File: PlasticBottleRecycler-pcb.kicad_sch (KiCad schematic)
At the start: 26 parts, among them J1 SWIM, J2 LCD, J3 Screw_Terminal_01x04, J4 NTC, J5 HEATER, J6 FAN1, J7 +12V, J8 +5V, Q1 IRF3205, Q2 BC337, SW1 RESET, SW2 SW_Push, SW3 SW_Push, SW4 SW_Push, U1 STM8S005K6T6C

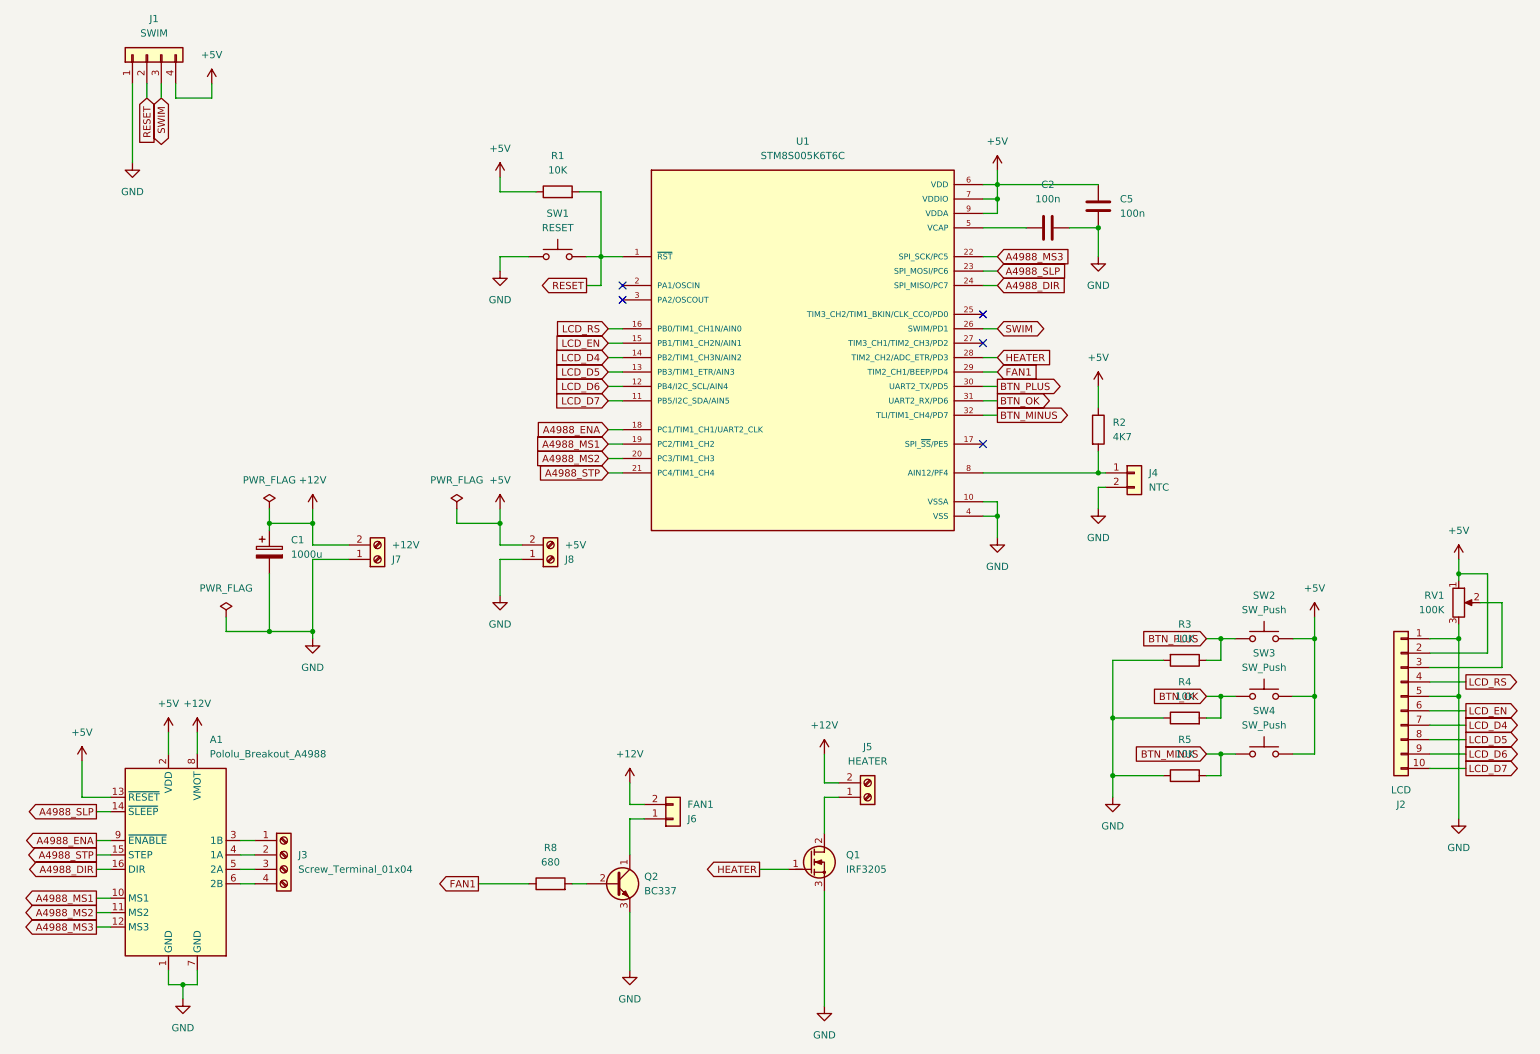
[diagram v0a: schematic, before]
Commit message: Revision 2.0
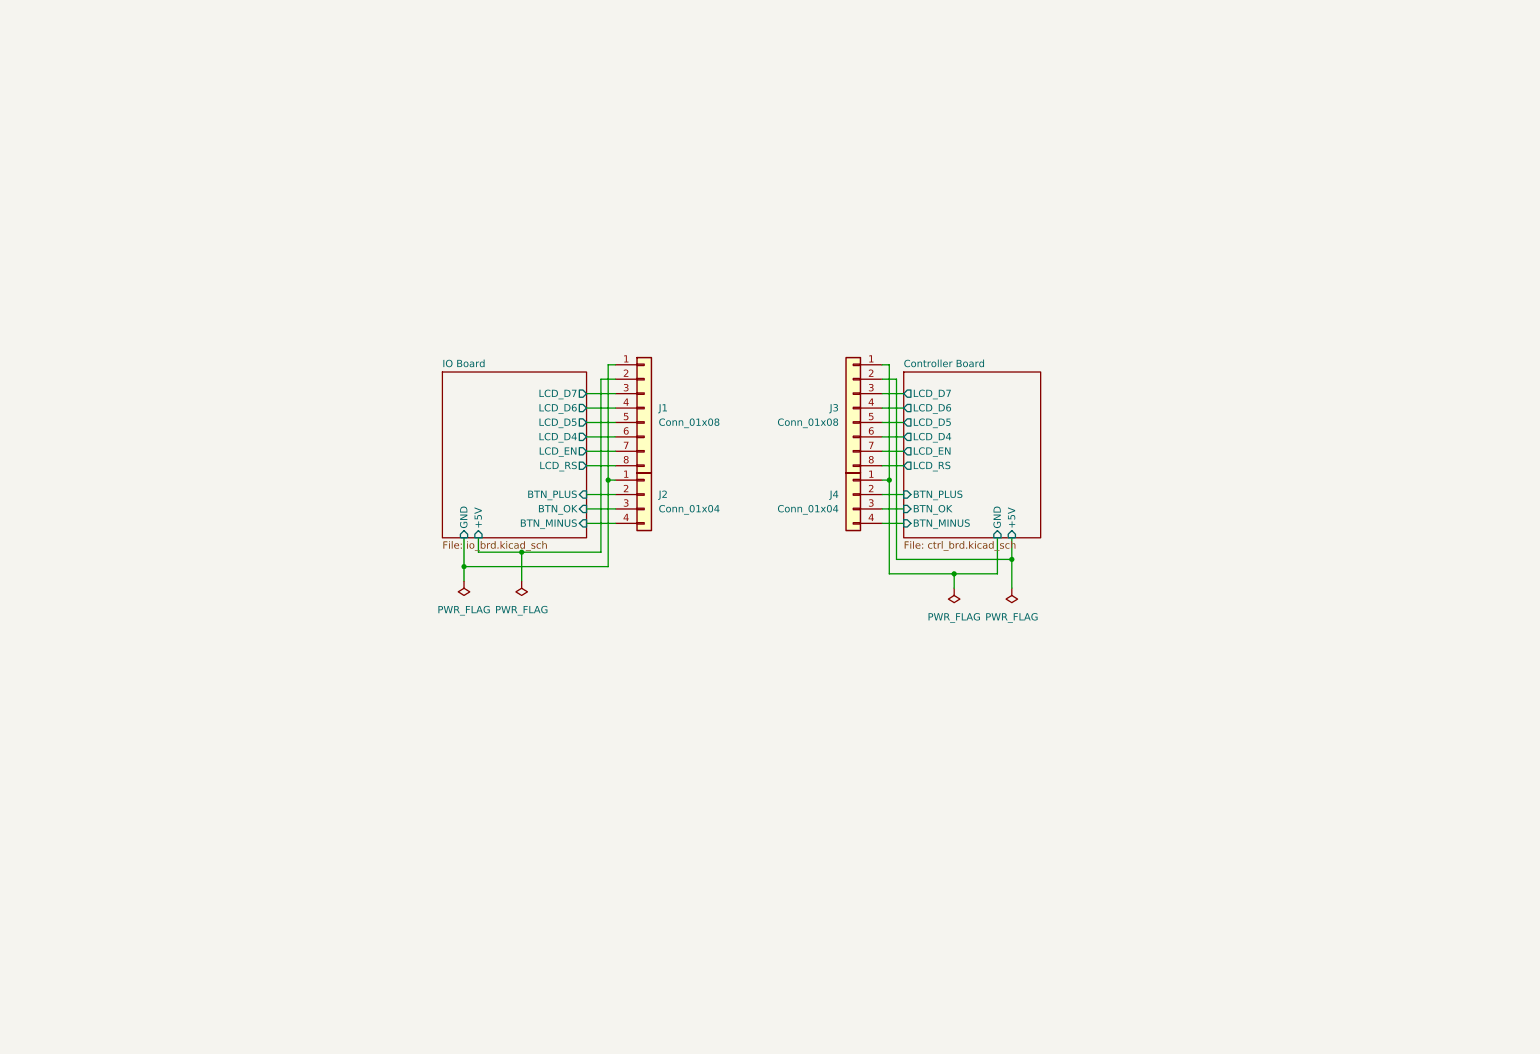
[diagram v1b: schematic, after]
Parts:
- removed A1: Pololu_Breakout_A4988, Module:Pololu_Breakout-16_15.2x20.3mm, symbol Driver_Motor:Pololu_Breakout_A4988
- removed C1: 1000u, Capacitor_THT:CP_Radial_D10.0mm_P5.00mm, symbol Device:C_Polarized
- removed C2, C5: 100n, Capacitor_THT:C_Disc_D6.0mm_W2.5mm_P5.00mm, symbol Device:C
- removed J1: SWIM, Connector_PinHeader_2.54mm:PinHeader_1x04_P2.54mm_Vertical, symbol Connector_Generic:Conn_01x04
- removed J2: LCD, Connector_PinHeader_2.54mm:PinHeader_1x10_P2.54mm_Vertical, symbol Connector_Generic:Conn_01x10
- removed J3: Screw_Terminal_01x04, TerminalBlock:TerminalBlock_bornier-4_P5.08mm, symbol Connector:Screw_Terminal_01x04
- removed J4: NTC, Connector_JST:JST_XH_B2B-XH-A_1x02_P2.50mm_Vertical, symbol Connector_Generic:Conn_01x02
- removed J5: HEATER, TerminalBlock:TerminalBlock_bornier-2_P5.08mm, symbol Connector:Screw_Terminal_01x02
- removed J6: FAN1, Connector_PinHeader_2.54mm:PinHeader_1x02_P2.54mm_Vertical, symbol Connector_Generic:Conn_01x02
- removed J7: +12V, TerminalBlock:TerminalBlock_bornier-2_P5.08mm, symbol Connector:Screw_Terminal_01x02
- removed J8: +5V, TerminalBlock:TerminalBlock_bornier-2_P5.08mm, symbol Connector:Screw_Terminal_01x02
- removed Q1: IRF3205, PCM_Package_TO_SOT_THT_AKL:TO-220-3_Vertical_GDS, symbol PCM_Transistor_MOSFET_AKL:IRF3205
- removed Q2: BC337, PCM_Package_TO_SOT_THT_AKL:TO-92_Inline_Wide_CBE, symbol PCM_Transistor_BJT_AKL:BC337
- removed R1, R3, R4, R5: 10K, Resistor_THT:R_Axial_DIN0204_L3.6mm_D1.6mm_P5.08mm_Horizontal, symbol Device:R
- removed R2: 4K7, Resistor_THT:R_Axial_DIN0204_L3.6mm_D1.6mm_P5.08mm_Horizontal, symbol Device:R
- removed R8: 680, Resistor_THT:R_Axial_DIN0207_L6.3mm_D2.5mm_P10.16mm_Horizontal, symbol Device:R
- removed RV1: 100K, Potentiometer_THT:Potentiometer_Vishay_T73YP_Vertical, symbol Device:R_Potentiometer
- removed SW1: RESET, Button_Switch_THT:SW_PUSH_6mm_H5mm, symbol Switch:SW_Push
- removed SW2, SW3, SW4: SW_Push, Button_Switch_THT:SW_PUSH_6mm_H5mm, symbol Switch:SW_Push
- removed U1: STM8S005K6T6C, Package_QFP:LQFP-32_7x7mm_P0.8mm, symbol Extras:STM8S005K6T6C
- added J1, J3: Conn_01x08, Connector_Molex:Molex_KK-254_AE-6410-08A_1x08_P2.54mm_Vertical, symbol Connector_Generic:Conn_01x08
- added J2, J4: Conn_01x04, Connector_Molex:Molex_KK-254_AE-6410-04A_1x04_P2.54mm_Vertical, symbol Connector_Generic:Conn_01x04
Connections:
- new net Controller Board/+5V: J3.2 (Pin_2)
- new net Controller Board/BTN_MINUS: J4.4 (Pin_4)
- new net Controller Board/BTN_OK: J4.3 (Pin_3)
- new net Controller Board/BTN_PLUS: J4.2 (Pin_2)
- new net Controller Board/GND: J3.1 (Pin_1), J4.1 (Pin_1)
- new net Controller Board/LCD_D4: J3.6 (Pin_6)
- new net Controller Board/LCD_D5: J3.5 (Pin_5)
- new net Controller Board/LCD_D6: J3.4 (Pin_4)
- new net Controller Board/LCD_D7: J3.3 (Pin_3)
- new net Controller Board/LCD_EN: J3.7 (Pin_7)
- new net Controller Board/LCD_RS: J3.8 (Pin_8)
- new net IO Board/+5V: J1.2 (Pin_2)
- new net IO Board/BTN_MINUS: J2.4 (Pin_4)
- new net IO Board/BTN_OK: J2.3 (Pin_3)
- new net IO Board/BTN_PLUS: J2.2 (Pin_2)
- new net IO Board/GND: J1.1 (Pin_1), J2.1 (Pin_1)
- new net IO Board/LCD_D4: J1.6 (Pin_6)
- new net IO Board/LCD_D5: J1.5 (Pin_5)
- new net IO Board/LCD_D6: J1.4 (Pin_4)
- new net IO Board/LCD_D7: J1.3 (Pin_3)
- new net IO Board/LCD_EN: J1.7 (Pin_7)
- new net IO Board/LCD_RS: J1.8 (Pin_8)
- no-connect marks 5 -> 0
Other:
- added sheet Controller Board (ctrl_brd.kicad_sch)
- added sheet IO Board (io_brd.kicad_sch)
